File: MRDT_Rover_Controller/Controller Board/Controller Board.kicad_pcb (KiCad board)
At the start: 2 copper layers, 137.6 x 81.5 mm, 32 parts, among them Q1 S8050, SW1 EG1218

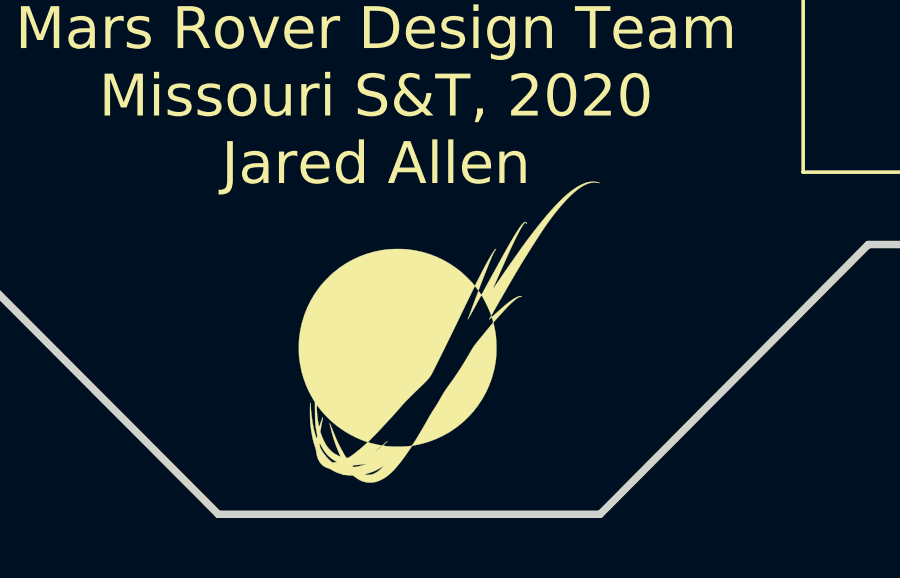
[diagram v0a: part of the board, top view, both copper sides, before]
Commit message: Silkscreen Updated
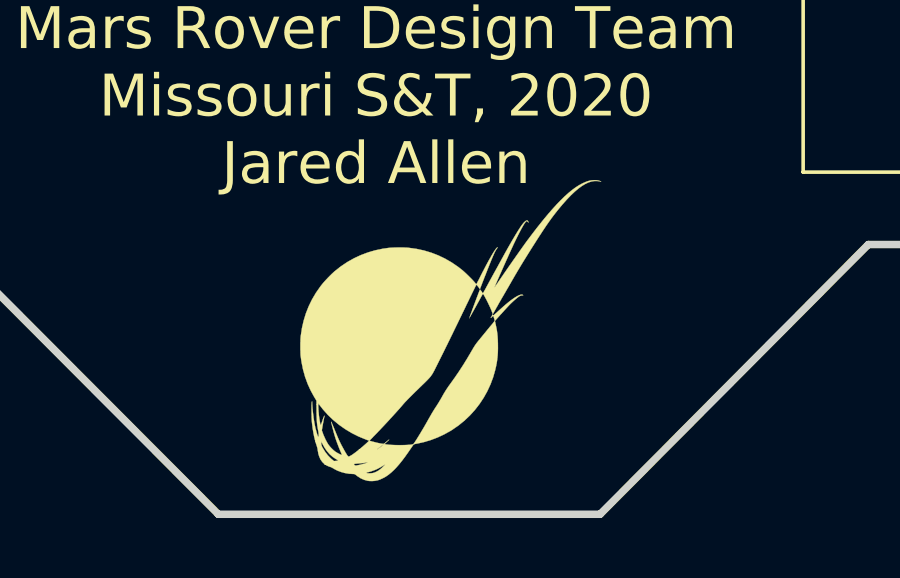
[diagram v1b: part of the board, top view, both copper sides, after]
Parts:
- moved G*** 0.07 mm to (92.7, 127.4)
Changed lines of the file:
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@@
   )
   (setup
-    (last_trace_width 0.381)
+    (last_trace_width 0.25)
     (user_trace_width 0.381)
     (user_trace_width 15)
@@
   )
   (module MRDT_Silkscreens:0_MRDT_Logo_10mm (layer F.Cu)
-    (at 92.6084 127.4572)
+    (at 92.6592 127.4064)
     (tags "Logo, MRDT")
     (fp_text reference G*** (at -1.143 6.4008) (layer Dwgs.User) hide
